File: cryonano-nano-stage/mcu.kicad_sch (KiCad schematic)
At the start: 18 parts, among them J8 Conn_ST_STDC14, U5 STM32L412CBT6P, U9 LP5817DRLR, Y1 Crystal

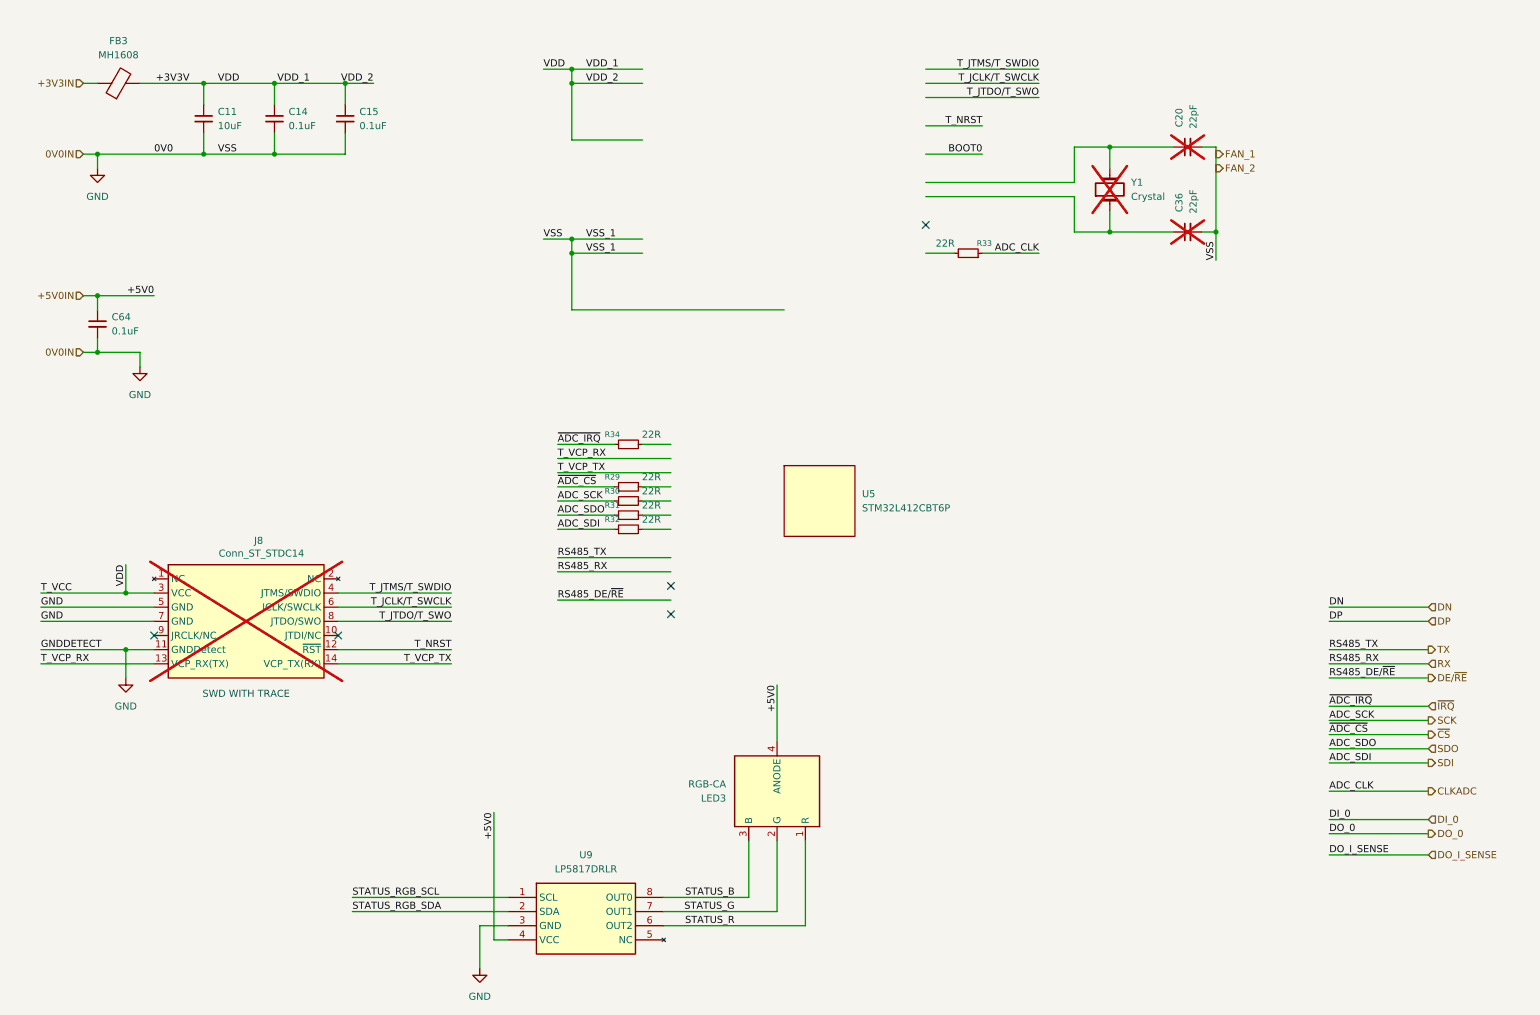
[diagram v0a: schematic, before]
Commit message: sch updated
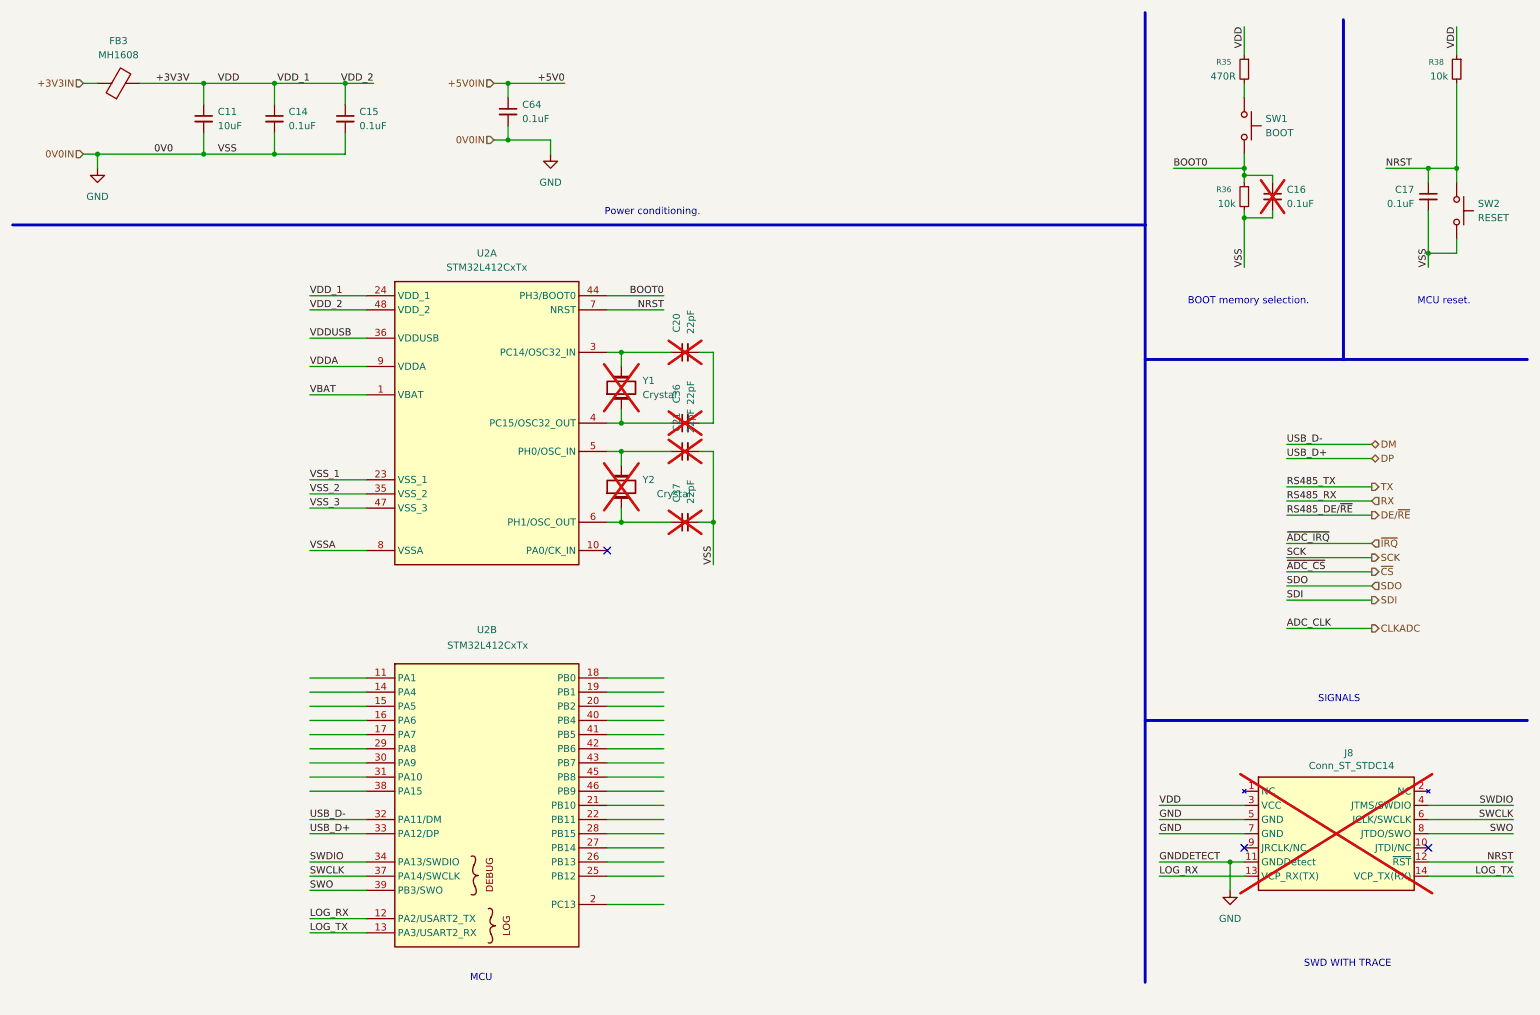
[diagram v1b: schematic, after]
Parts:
- removed LED3: RGB-CA, footprints:19037ARSGHBHW1S032T, symbol symbols:19-037A_RSGHBHW1-S03_2T
- removed R29, R30, R31, R32, R33, R34: 22R, Resistor_SMD:R_0603_1608Metric, symbol Device:R_Small
- removed U5: STM32L412CBT6P, Package_QFP:LQFP-32_7x7mm_P0.8mm, symbol symbols:STM32L412CBT6P
- removed U9: LP5817DRLR, footprints:LP5817DRLR, symbol symbols:LP5817DRLR
- added C16, C17: 0.1uF, Capacitor_SMD:C_0603_1608Metric, symbol Device:C_Small
- added C21, C37: 22pF, Capacitor_SMD:C_0603_1608Metric, symbol Device:C_Small
- added R35: 470R, Resistor_SMD:R_0603_1608Metric, symbol Device:R_Small
- added R36, R38: 10k, Resistor_SMD:R_0603_1608Metric, symbol Device:R_Small
- added SW1: BOOT, symbol Switch:SW_Push
- added SW2: RESET, symbol Switch:SW_Push
- added U2: STM32L412CxTx, QFP50P900X900X160-48N, symbol symbols:STM32L412CxTx
- added Y2: Crystal, Crystal:Crystal_SMD_3215-2Pin_3.2x1.5mm, symbol Device:Crystal
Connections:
- net +3V3V: now also R35.1, R38.1, U2.24 (VDD_1), U2.48 (VDD_2)
- net BOOT0: now also C16.1, R36.1, SW1.2, U2.44 (PH3/BOOT0)
- net DP: now also U2.33 (PA12/DP)
- net GND: now also C16.2, C17.2, C21.2, C37.2, R36.2, SW2.2; no longer C20.2, C36.2
- net at C36.1, Y1.1: now also U2.4 (PC15/OSC32_OUT)
- net at C20.1, Y1.2: now also U2.3 (PC14/OSC32_IN)
- net T_JCLK/T_SWCLK renamed SWCLK
- net SWCLK: now also U2.37 (PA14/SWCLK)
- net T_JTDO/T_SWO renamed SWO
- net SWO: now also U2.39 (PB3/SWO)
- net T_JTMS/T_SWDIO  renamed SWDIO
- net SWDIO: now also U2.34 (PA13/SWDIO)
- net T_NRST renamed NRST
- net NRST: now also C17.1, R38.2, SW2.1, U2.7 (NRST)
- net T_VCP_RX renamed LOG_RX
- net LOG_RX: now also U2.12 (PA2/USART2_TX)
- net T_VCP_TX renamed LOG_TX
- net LOG_TX: now also U2.13 (PA3/USART2_RX)
- new net: C20.2, C36.2
- new net: C37.1, U2.6 (PH1/OSC_OUT), Y2.1
- new net: C21.1, U2.5 (PH0/OSC_IN), Y2.2
- new net: R35.2, SW1.1
- new net DM: U2.32 (PA11/DM)
- new net VBAT: U2.1 (VBAT)
- new net VDDA: U2.9 (VDDA)
- new net VDDUSB: U2.36 (VDDUSB)
- new net VSSA: U2.8 (VSSA)
- new net VSS_1: U2.23 (VSS_1)
- new net VSS_2: U2.35 (VSS_2)
- new net VSS_3: U2.47 (VSS_3)
- no-connect marks 5 -> 3
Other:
- note added: "BOOT memory selection."
- note added: "MCU"
- note added: "MCU reset."
- note added: "Power conditioning."
- note added: "SIGNALS"
- moved on the sheet: C20, C36, C64, J8, Y1
